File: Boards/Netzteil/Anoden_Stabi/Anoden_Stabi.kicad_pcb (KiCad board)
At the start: 2 copper layers, 100 x 80 mm, 26 parts, among them P1 CONN_4, P2 CONN_2, P3 CONN_2, P4 CONN_2, Q1 2SC2979, Q2 MJE5731

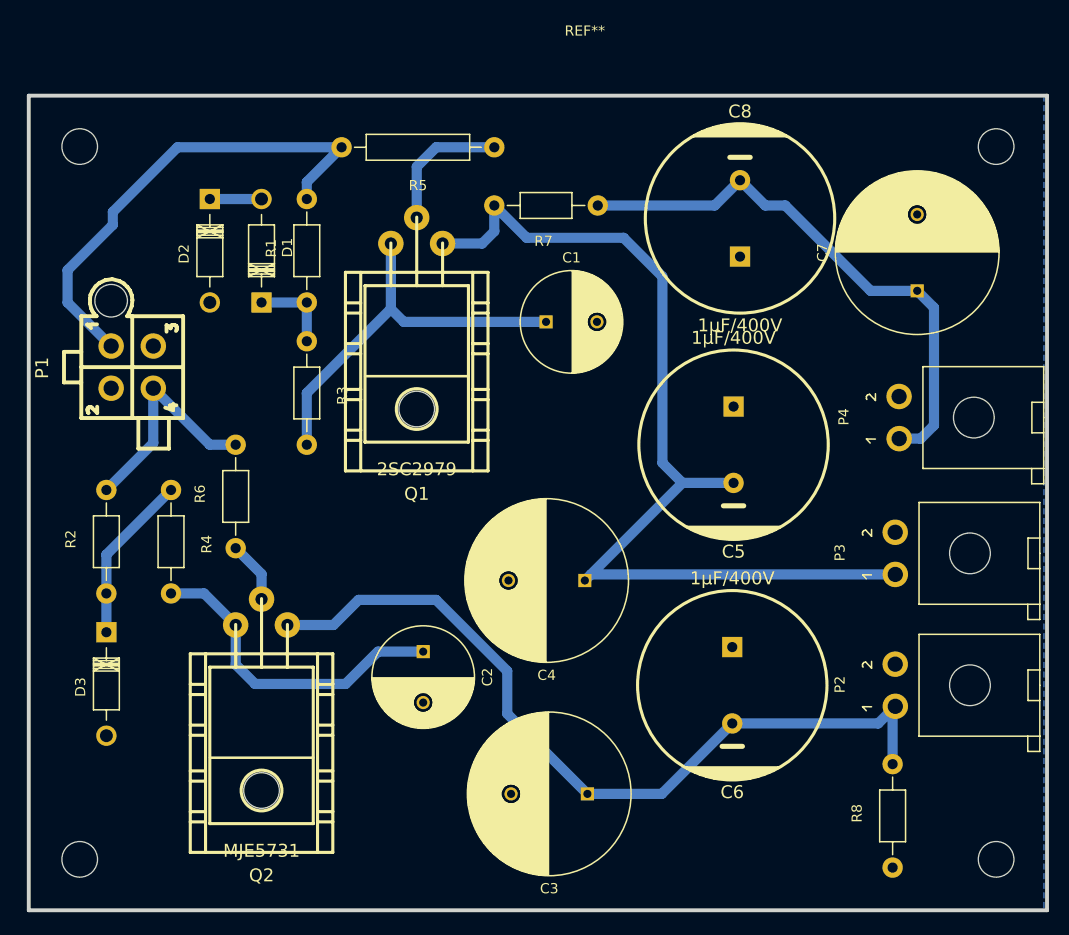
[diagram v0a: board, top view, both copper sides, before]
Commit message: Layouting...
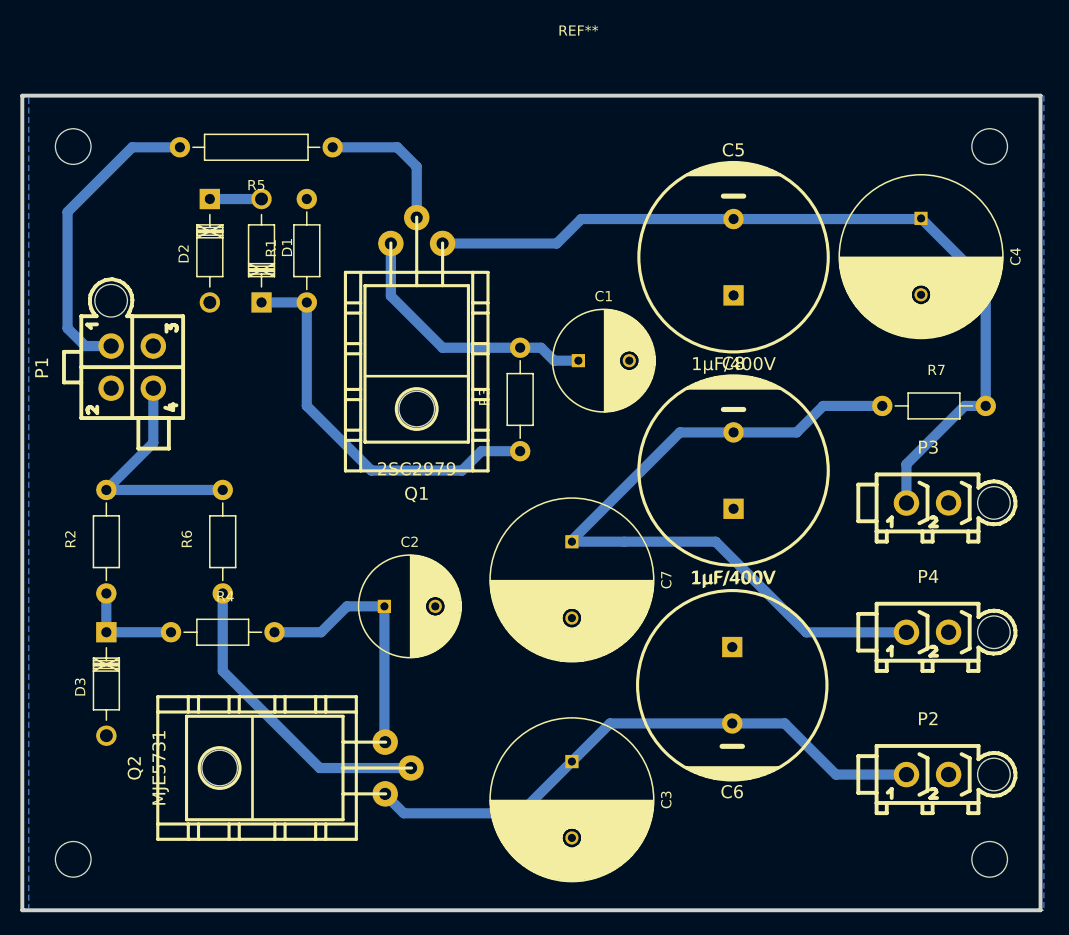
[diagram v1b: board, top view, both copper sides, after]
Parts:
- removed R8: 30k, Resistors_ThroughHole:Resistor_Horizontal_RM10mm
- P2, P3, P4: footprint Sockets_Mini-Universal:MiniUniversalMate-N-LokSocket_2PinHorizontal -> MiniUniversalMate-N-LokSockets_13Aug2012:MiniUniversalMate-N-LokSocket_2PinVertical_12Aug2012
- moved C4 48.5 mm to (163.8, 60.3), turned to 270 degrees
- moved C7 41.9 mm to (129.5, 92.1), turned to 270 degrees
- moved R7 34.2 mm to (160.0, 78.7), turned to 0 degrees
- moved C8 24.8 mm to (145.4, 85.1)
- moved R3 23.6 mm to (124.5, 83.2), turned to 90 degrees
- moved P4 21.3 mm to (164.5, 101.0), turned to 0 degrees
- moved C5 18.4 mm to (145.4, 64.1), turned to 0 degrees
- moved R5 15.9 mm to (106.0, 53.3)
- moved R4 14.0 mm to (90.2, 101.0), turned to 0 degrees
- moved P2 9.32 mm to (164.5, 114.9), turned to 0 degrees
- moved Q2 6.87 mm to (102.9, 114.3), turned to 90 degrees
- moved P3 5.88 mm to (164.5, 88.3), turned to 0 degrees
- moved C2 5.85 mm to (111.1, 98.4), turned to 0 degrees
- moved C1 4.96 mm to (130.2, 74.3)
- moved R6 4.62 mm to (95.2, 97.2)
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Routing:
- net Net-(D1-Pad1): track 8.26 -> 39.0 mm
- net Net-(Q2-Pad2): track 6.06 -> 30.1 mm
- net -120V: track 80.4 -> 57.8 mm
- net +450V: track 48.4 -> 30.1 mm
- net +240V: track 54.7 -> 72.6 mm
- net +300V: track 97.9 -> 83.1 mm
- net Net-(C1-Pad1): track 38.9 -> 26.2 mm
- net Net-(C2-Pad1): track 32.0 -> 25.2 mm
- net Net-(D3-Pad1): track 16.6 -> 10.2 mm
- net -180V: track 22.3 -> 23.3 mm
- net Net-(Q1-Pad2): track 13.4 -> 14.0 mm

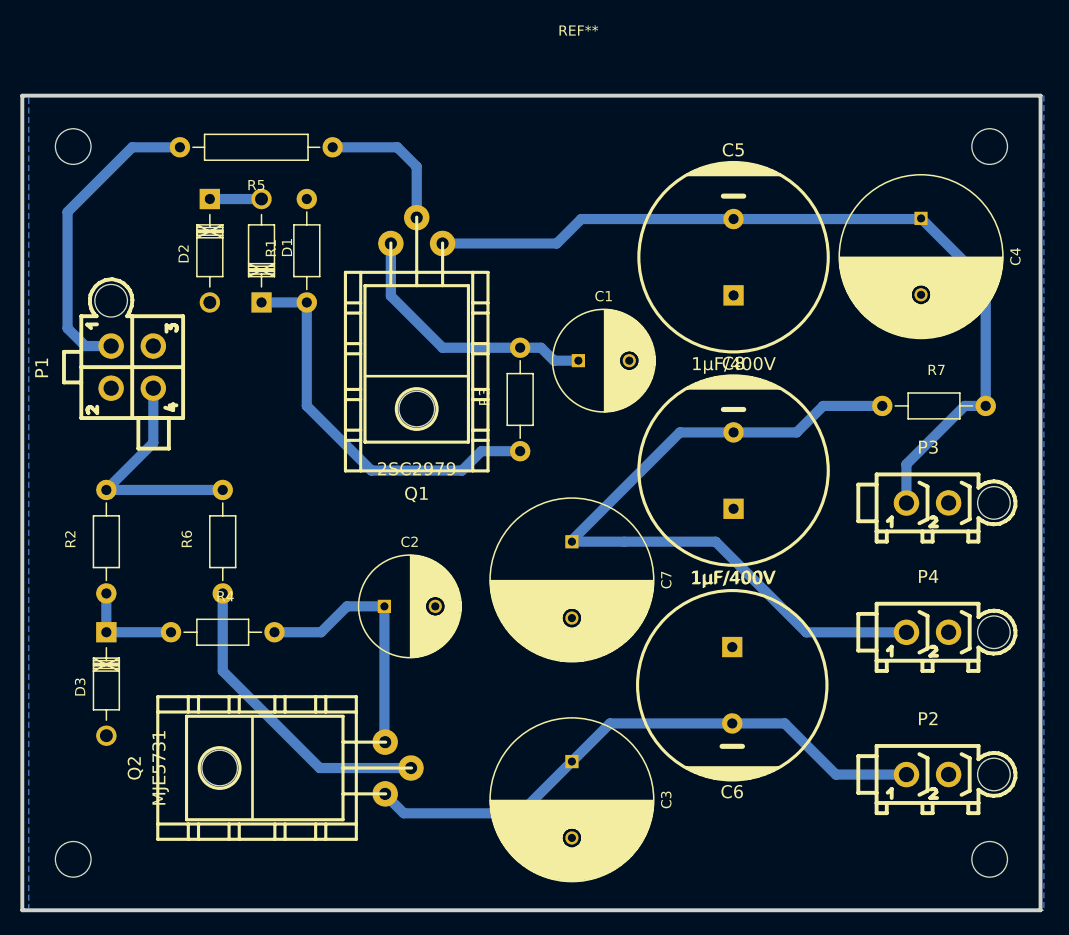
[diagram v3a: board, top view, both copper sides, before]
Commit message: Work in Progress
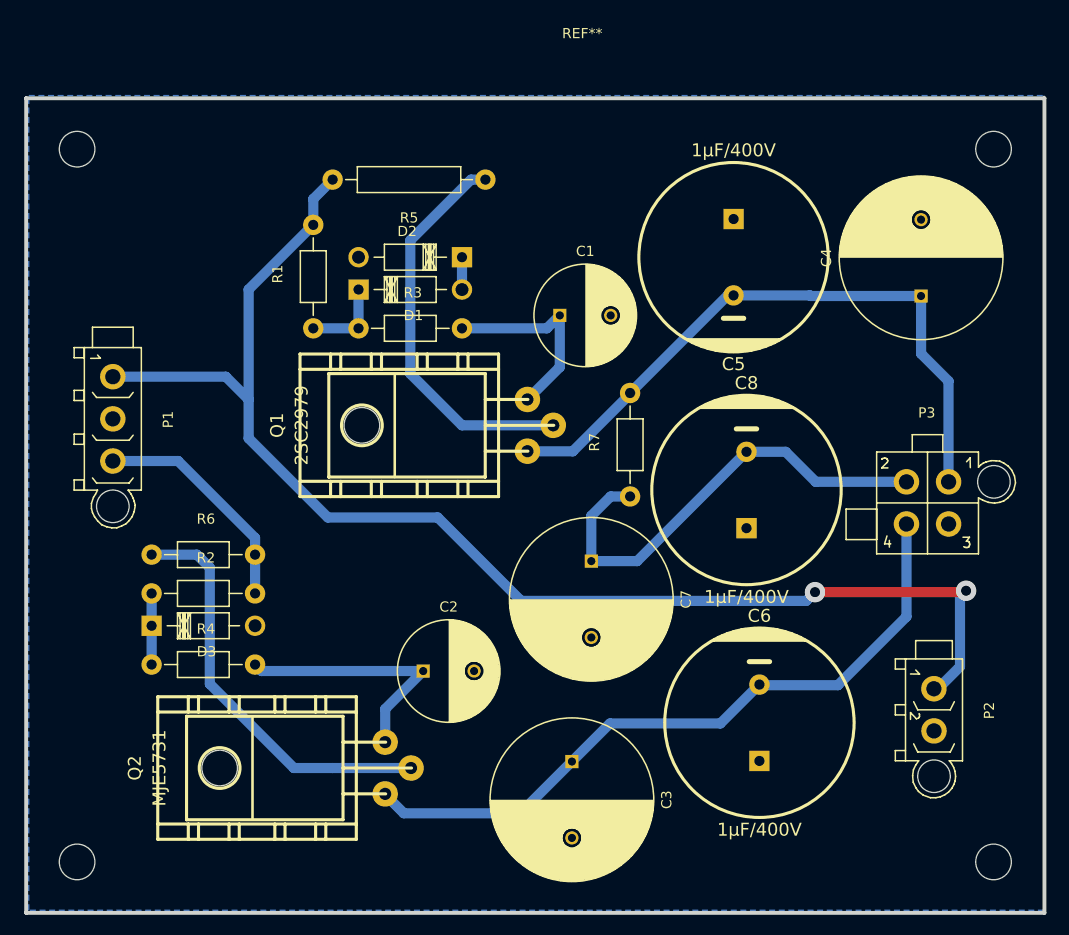
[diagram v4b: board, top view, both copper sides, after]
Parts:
- removed P4: CONN_2, MiniUniversalMate-N-LokSockets_13Aug2012:MiniUniversalMate-N-LokSocket_2PinVertical_12Aug2012
- P1: value CONN_4 -> CONN_3; footprint MiniUniversalMate-N-LokSockets_13Aug2012:MiniUniversalMate-N-LokSocket_4PinVertical_13Aug2012 -> Connectors_Mini-Universal:MiniUniversalMate-N-LokSocket_3PinVertical
- P2: footprint MiniUniversalMate-N-LokSockets_13Aug2012:MiniUniversalMate-N-LokSocket_2PinVertical_12Aug2012 -> Connectors_Mini-Universal:MiniUniversalMate-N-LokSocket_2PinVertical
- P3: value CONN_2 -> CONN_4; footprint MiniUniversalMate-N-LokSockets_13Aug2012:MiniUniversalMate-N-LokSocket_2PinVertical_12Aug2012 -> Connectors_Mini-Universal:MiniUniversalMate-N-LokSocket_4PinVertical
- moved R7 26.3 mm to (135.3, 87.6), turned to 90 degrees
- moved D2 25.4 mm to (118.7, 64.1), turned to 180 degrees
- moved R3 19.9 mm to (108.6, 71.1), turned to 0 degrees
- moved R5 15.3 mm to (121.0, 56.5)
- moved Q1 9.86 mm to (116.8, 80.6), turned to 90 degrees
- moved D1 9.61 mm to (108.6, 67.3), turned to 0 degrees
- moved R6 7.96 mm to (88.3, 93.3), turned to 0 degrees
- moved C4 7.62 mm to (163.8, 67.9), turned to 90 degrees
- moved C2 7.41 mm to (114.9, 104.8)
- moved P2 6.38 mm to (165.1, 108.6), turned to 270 degrees
- moved P1 5.43 mm to (84.5, 80.0), turned to 270 degrees
- moved C1 4.81 mm to (128.3, 69.8)
- moved C6 4.55 mm to (148.0, 109.9), turned to 0 degrees
- moved D3 4.49 mm to (88.3, 100.3), turned to 0 degrees
- moved R2 4.45 mm to (88.3, 97.2), turned to 0 degrees
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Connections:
- P1 pad 3: GND -> -180V
- P2 pad 1: -120V -> +450V
- P3 pad 2: GND -> +240V
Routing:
- net +450V: track 30.1 -> 131.7 mm, vias 0 -> 2
- net Net-(D1-Pad1): track 39.0 -> 8.25 mm
- net +240V: track 72.6 -> 45.7 mm
- net Net-(Q1-Pad2): track 14.0 -> 39.1 mm
- net +300V: track 83.1 -> 64.6 mm
- net -120V: track 57.8 -> 69.2 mm
- net Net-(Q2-Pad2): track 30.1 -> 40.9 mm
- net Net-(C1-Pad1): track 26.2 -> 19.8 mm
- net Net-(D3-Pad1): track 10.2 -> 6.98 mm
- net Net-(D1-Pad2): track 5.07 -> 3.17 mm
- net -180V: track 23.3 -> 22.6 mm
